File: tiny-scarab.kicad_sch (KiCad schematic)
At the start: 22 parts, among them J1 Conn_02x07_Odd_Even, J2 Conn_01x05_Pin, J4 Conn_02x07_Odd_Even, J5 Screw_Hole, J6 Screw_Hole, J7 Screw_Hole, J8 Screw_Hole, Q3 IRLML2502TRPBF, SW4 SLW-883935-2A-D, SW5 PTS636_SL43_SMTR_LFS, U1 CH32V003F4P6

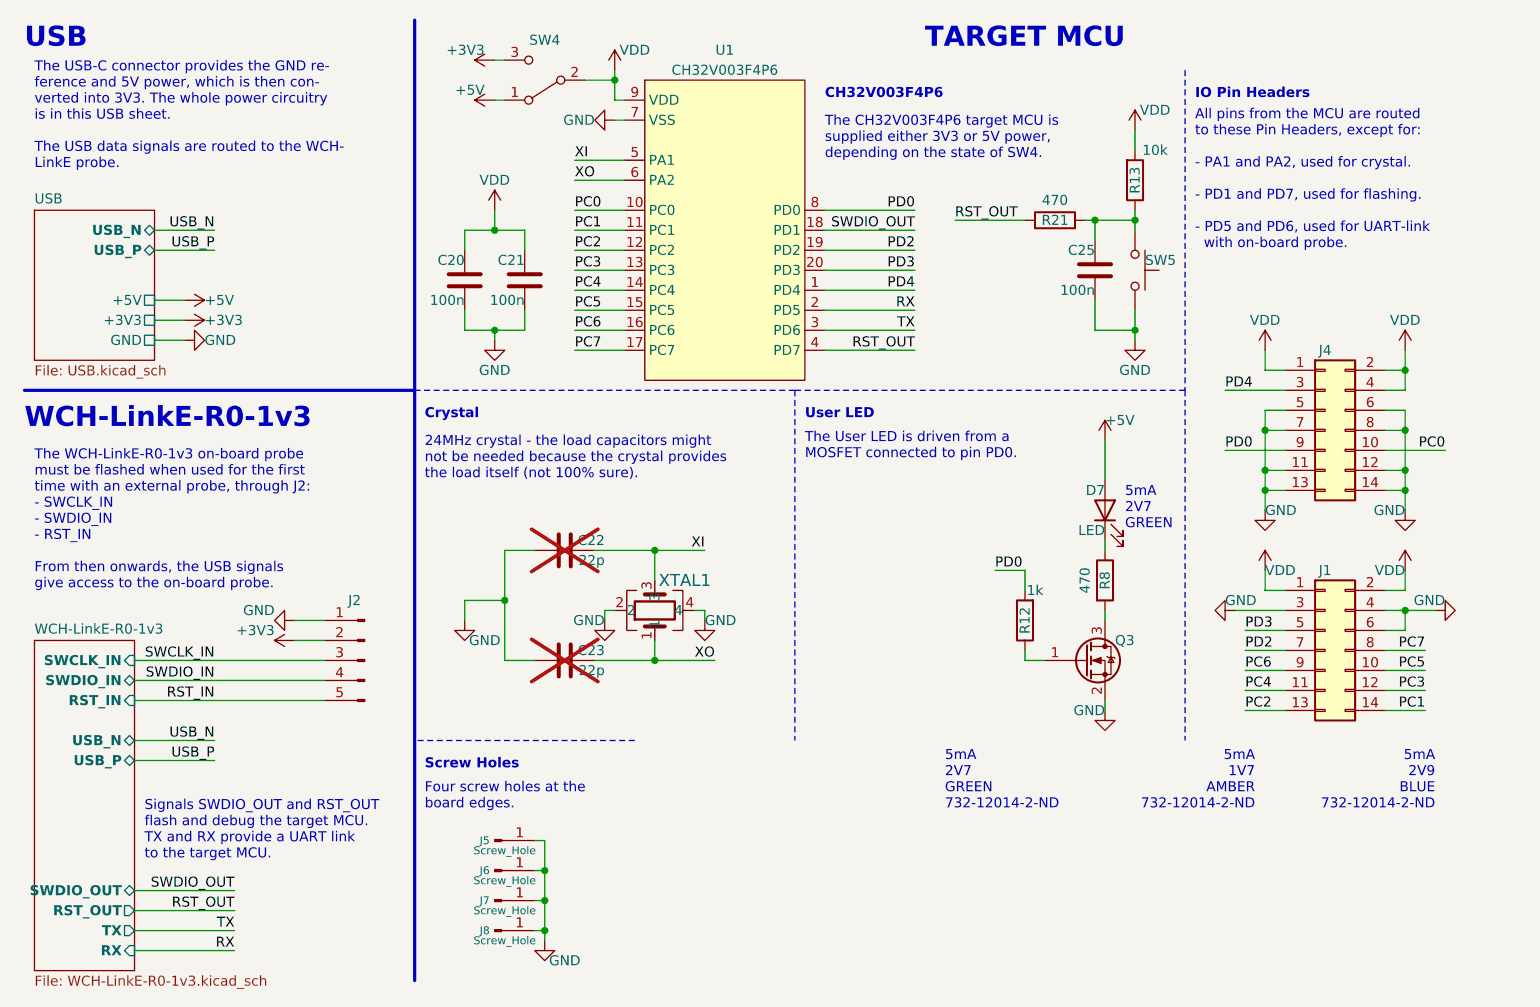
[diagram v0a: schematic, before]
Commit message: Improve layout
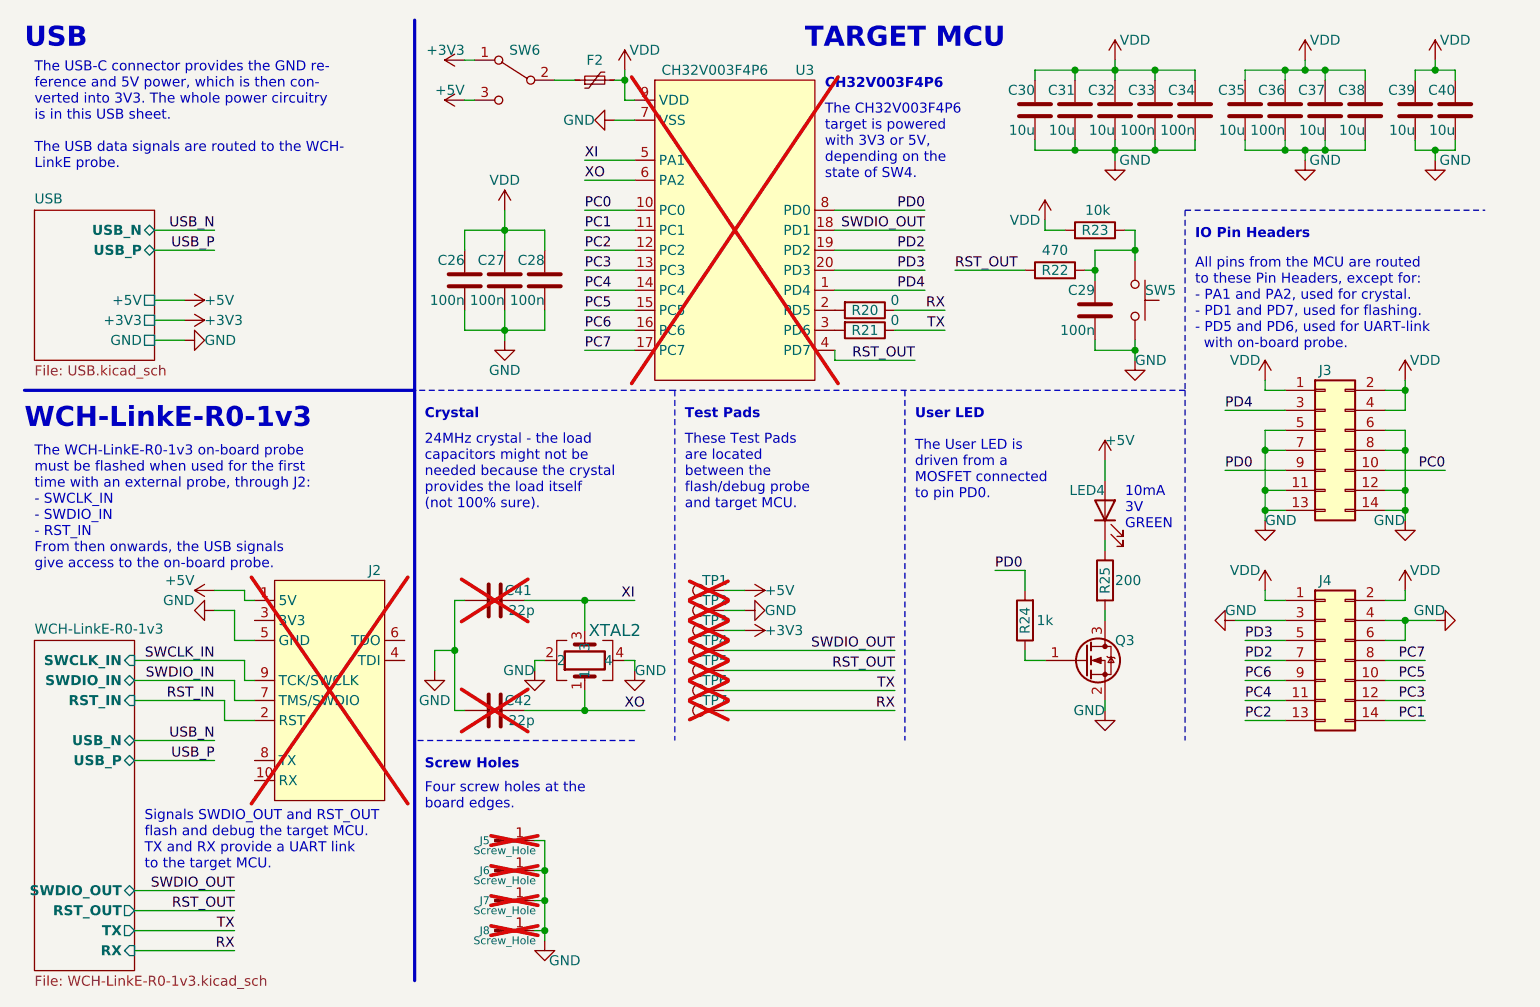
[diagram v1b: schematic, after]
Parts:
- removed J2: Conn_01x05_Pin, Tiny_Scarab:PinHeader_1x05_P2.54mm_Vertical, symbol Tiny_Scarab:Conn_01x05_Pin
- removed SW4: SLW-883935-2A-D, Tiny_Scarab:SLW-883935-2A-D, symbol Tiny_Scarab:SLW-883935-2A-D
- added C26, C33, C34, C36: 100n, Capacitor_SMD:C_0402_1005Metric_Pad0.74x0.62mm_HandSolder, symbol Device:C
- added C30, C31, C32, C35, C37, C38, C39, C40: 10u, Capacitor_SMD:C_0805_2012Metric, symbol Device:C
- added F2: 0402L050SLKR, Tiny_Scarab:0402L050SLKR, symbol Device:Polyfuse_Small
- added J2: ~, Tiny_Scarab:Tag-Connect_TC2050-IDC-NL_2x05_P1.27mm_Vertical_with_bottom_clip, symbol Tiny_Scarab:TC2050-IDC-NL-WCH-LinkE-R0-1v3
- added R20, R21: 0, Resistor_SMD:R_0402_1005Metric_Pad0.72x0.64mm_HandSolder, symbol Device:R
- added SW6: SLW-883935-2A-D, Tiny_Scarab:SLW-883935-2A-D, symbol Tiny_Scarab:SLW-883935-2A-D
- added TP1, TP2, TP3, TP4, TP5, TP6, TP7: TestPoint, Tiny_Scarab:TestPoint_Pad_D1.0mm, symbol Connector:TestPoint
- C27: renamed from C20; GPN GPC0402104-25 -> (none); MPN (none) -> GPC0402104-25
- C28: renamed from C21; GPN GPC0402104-25 -> (none); MPN (none) -> GPC0402104-25
- C29: renamed from C25; GPN GPC0402104-25 -> (none); MPN (none) -> GPC0402104-25
- C41: renamed from C22; GPN GPC0402220 -> (none); MPN (none) -> GPC0402220; now left out of the parts list
- C42: renamed from C23; GPN GPC0402220 -> (none); MPN (none) -> GPC0402220; now left out of the parts list
- J5, J6, J7, J8: now not fitted; now left out of the parts list
- Q3: DPN IRLML2502TRPBFTR-ND -> (none); Distributor DigiKey -> (none); SPN (none) -> IRLML2502TRPBFTR-ND; Supplier (none) -> DigiKey
- R22: renamed from R21; GPN GPR0402470R -> (none); MPN (none) -> GPR0402470R
- R23: renamed from R13; GPN GPR040210K -> (none); MPN (none) -> GPR040210K
- R24: renamed from R12; GPN GPR04021K -> (none); MPN (none) -> GPR04021K
- R25: renamed from R8; value 470 -> 200; GPN GPR0402470R -> (none); MPN (none) -> GPR0402200R
- U3: renamed from U1; now not fitted; now left out of the parts list
- renumbered J4 to J3, J1 to J4, D7 to LED4, XTAL1 to XTAL2
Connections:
- net +3V3: now also SW6.1 (A), TP3.1
- net +5V: now also J2.1 (5V), SW6.3 (C), TP1.1
- net GND: now also C26.2, C30.2, C31.2, C32.2, C33.2, C34.2, C35.2, C36.2, C37.2, C38.2, C39.2, C40.2, J2.5 (GND), TP2.1
- net RST_IN: now also J2.2 (RST)
- net RST_OUT: now also TP5.1
- net RX: now also R20.1, TP7.1; no longer U3.2 (PD5)
- net SWCLK_IN: now also J2.9 (TCK/SWCLK)
- net SWDIO_IN: now also J2.7 (TMS/SWDIO)
- net SWDIO_OUT: now also TP4.1
- net TX: now also R21.1, TP6.1; no longer U3.3 (PD6)
- net VDD: now also C26.1, C30.1, C31.1, C32.1, C33.1, C34.1, C35.1, C36.1, C37.1, C38.1, C39.1, C40.1, F2.2
- new net: F2.1, SW6.2 (B)
- new net: R20.2, U3.2 (PD5)
- new net: R21.2, U3.3 (PD6)
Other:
- note added: "10mA 3V GREEN"
- note added: "Test Pads"
- note added: "The CH32V003F4P6 target is powered with 3V3 or 5V, depending on the state of SW4."
- note added: "These Test Pads are located between the flash/debug probe and target MCU."
- note removed: "5mA 1V7 AMBER 732-12014-2-ND"
- note removed: "5mA 2V7 GREEN"
- note removed: "5mA 2V7 GREEN 732-12014-2-ND"
- note removed: "5mA 2V9 BLUE 732-12014-2-ND"
- note removed: "The CH32V003F4P6 target MCU is supplied either 3V3 or 5V power, depending on the state of SW4."
- moved on the sheet: C27, C28, C29, C41, C42, J3, J4, R22, R23, SW5, XTAL2

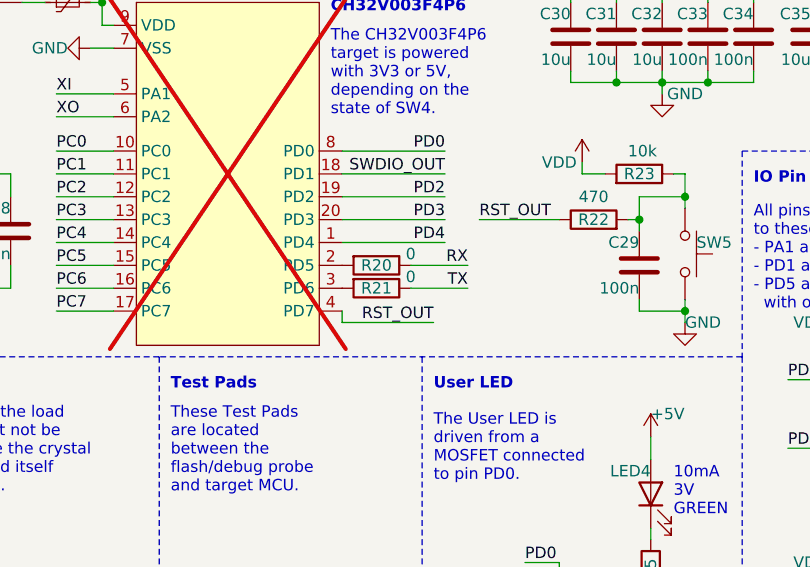
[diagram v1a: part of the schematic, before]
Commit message: Update design
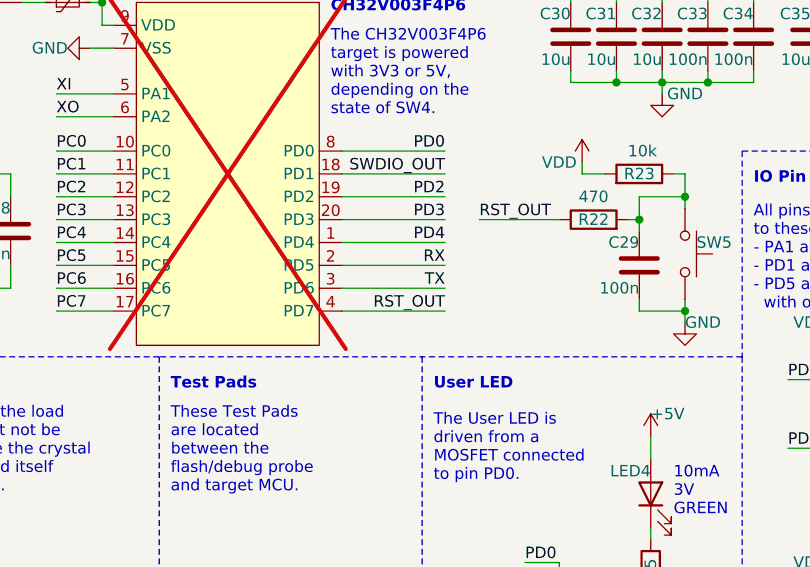
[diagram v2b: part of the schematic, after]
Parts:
- removed R20, R21: 0, Resistor_SMD:R_0402_1005Metric_Pad0.72x0.64mm_HandSolder, symbol Device:R
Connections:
- net RX: now also U3.2 (PD5)
- net TX: now also U3.3 (PD6)
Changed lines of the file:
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@@
-    (stroke (width 0) (type default))
-  )
-  (wire (pts (xy 123.19 49.53) (xy 129.54 49.53))
     (stroke (width 0) (type default))
   )
@@
     (stroke (width 0) (type dash))
   )
+  (wire (pts (xy 115.57 52.07) (xy 127 52.07))
+    (stroke (width 0) (type default))
+  )
   (wire (pts (xy 167.64 29.21) (xy 172.72 29.21))
     (stroke (width 0) (type default))
@@
     (stroke (width 0) (type default))
   )
-  (wire (pts (xy 115.57 55.88) (xy 125.73 55.88))
+  (wire (pts (xy 115.57 54.61) (xy 127 54.61))
     (stroke (width 0) (type default))
   )
@@
     (stroke (width 0) (type default))
   )
-  (wire (pts (xy 115.57 55.88) (xy 115.57 54.61))
+  (wire (pts (xy 115.57 49.53) (xy 127 49.53))
     (stroke (width 0) (type default))
   )
@@
     (stroke (width 0) (type default))
   )
-  (wire (pts (xy 123.19 52.07) (xy 129.54 52.07))
-    (stroke (width 0) (type default))
-  )
   (wire (pts (xy 185.42 93.98) (xy 190.5 93.98))
     (stroke (width 0) (type default))
@@
     (effects (font (size 1.27 1.27)) (justify left bottom))
   )
-  (label "RX" (at 129.54 49.53 180) (fields_autoplaced)
-    (effects (font (size 1.27 1.27)) (justify right bottom))
-  )
-  (label "RST_OUT" (at 125.73 55.88 180) (fields_autoplaced)
+  (label "RX" (at 127 49.53 180) (fields_autoplaced)
+    (effects (font (size 1.27 1.27)) (justify right bottom))
+  )
+  (label "RST_OUT" (at 127 54.61 180) (fields_autoplaced)
     (effects (font (size 1.27 1.27)) (justify right bottom))
   )
@@
     (effects (font (size 1.27 1.27)) (justify right bottom))
   )
-  (label "TX" (at 129.54 52.07 180) (fields_autoplaced)
+  (label "TX" (at 127 52.07 180) (fields_autoplaced)
     (effects (font (size 1.27 1.27)) (justify right bottom))
   )
@@
     )
   )
-  (symbol (lib_id "Device:R") (at 119.38 49.53 270) (unit 1)
-    (in_bom yes) (on_board yes) (dnp no)
-    (property "Reference" "R20" (at 119.38 49.53 90)
-      (effects (font (size 1.27 1.27)))
-    )
-    (property "Value" "0" (at 123.19 48.26 90)
-      (effects (font (size 1.27 1.27)))
-    )
-    (property "Footprint" "Resistor_SMD:R_0402_1005Metric_Pad0.72x0.64mm_HandSolder" (at 119.38 47.752 90)
-      (effects (font (size 1.27 1.27)) hide)
-    )
-    (property "Datasheet" "~" (at 119.38 49.53 0)
-      (effects (font (size 1.27 1.27)) hide)
-    )
-    (property "MPN" "GPR02010R" (at 119.38 49.53 0)
-      (effects (font (size 1.27 1.27)) hide)
-    )
-    (pin "2")
-    (pin "1")
-    (instances
-      (project "tiny-scarab"
-        (path "/156c5422-ee07-49a4-8263-a2dbd26b90bd"
-          (reference "R20") (unit 1)
-        )
-      )
-    )
-  )
   (symbol (lib_id "Connector:TestPoint") (at 101.6 95.25 90) (unit 1)
     (in_bom no) (on_board yes) (dnp yes)
@@
         )
       )
-    )
-  )
-  (symbol (lib_id "Device:R") (at 119.38 52.07 270) (unit 1)
-    (in_bom yes) (on_board yes) (dnp no)
-    (property "Reference" "R21" (at 119.38 52.07 90)
-      (effects (font (size 1.27 1.27)))
-    )
-    (property "Value" "0" (at 123.19 50.8 90)
-      (effects (font (size 1.27 1.27)))
-    )
-    (property "Footprint" "Resistor_SMD:R_0402_1005Metric_Pad0.72x0.64mm_HandSolder" (at 119.38 50.292 90)
-      (effects (font (size 1.27 1.27)) hide)
-    )
-    (property "Datasheet" "~" (at 119.38 52.07 0)
-      (effects (font (size 1.27 1.27)) hide)
-    )
-    (property "MPN" "GPR02010R" (at 119.38 52.07 0)
-      (effects (font (size 1.27 1.27)) hide)
-    )
-    (pin "2")
-    (pin "1")
-    (instances
-      (project "tiny-scarab"
-        (path "/156c5422-ee07-49a4-8263-a2dbd26b90bd"
-          (reference "R21") (unit 1)
-        )
-      )
